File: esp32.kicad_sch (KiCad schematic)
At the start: 28 parts, among them U26 SRV05-4, U4 W25Q128, U5 ESP32-S3, Y1 40MHz

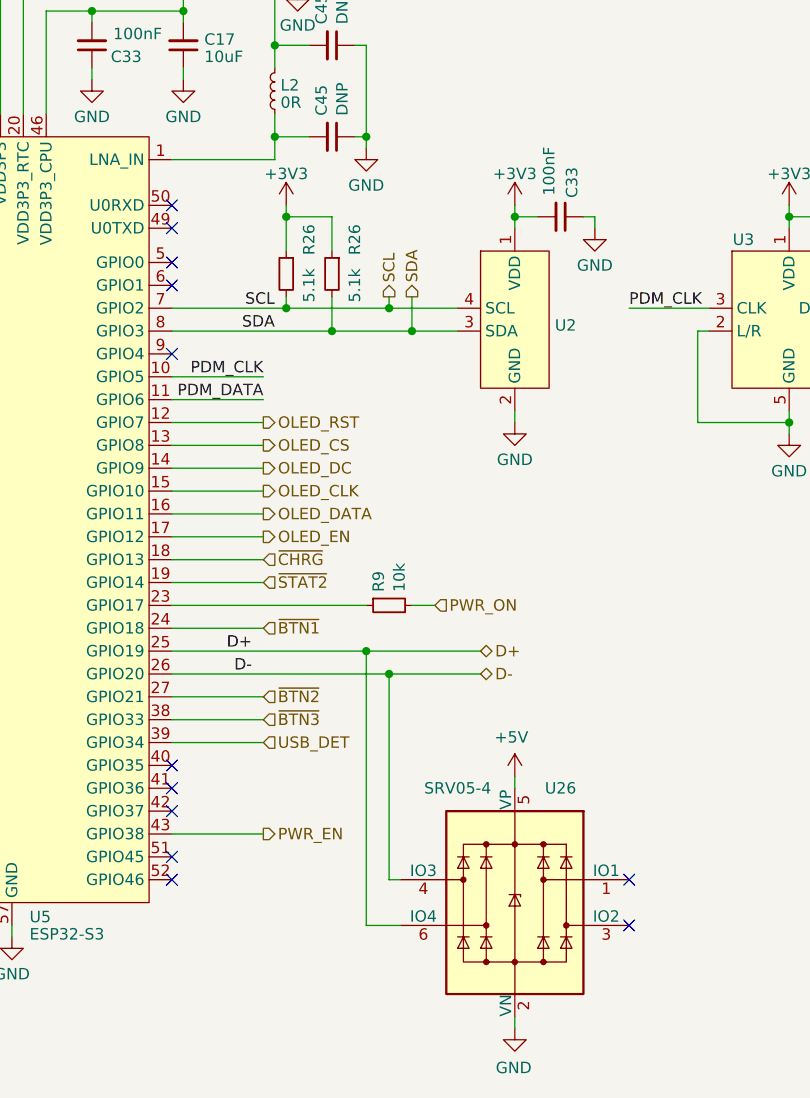
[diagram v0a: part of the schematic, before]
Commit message: Finish ESP32 fanout
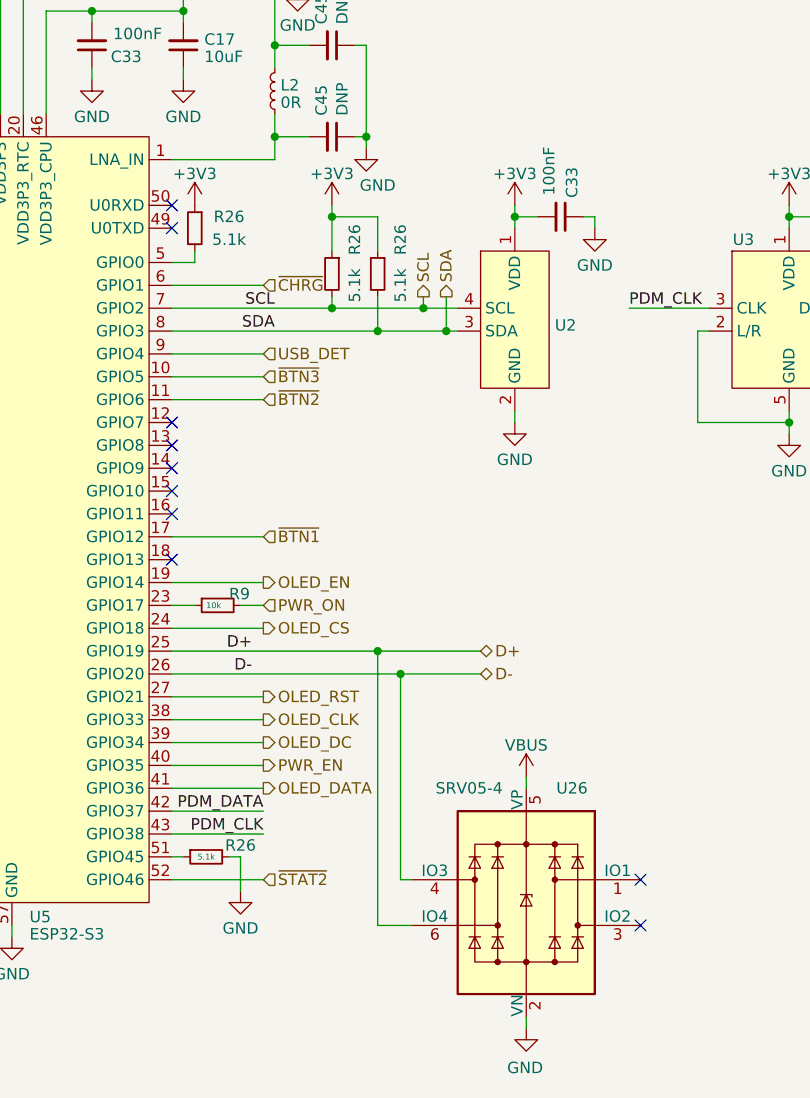
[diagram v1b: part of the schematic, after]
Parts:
- added R26 (x2): 5.1k, Resistor_SMD:R_0402_1005Metric, symbol Device:R_Small
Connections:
- net +3V3: now also R26.1
- net GND: now also R26.2
- net OLED_CLK: now also U5.38 (GPIO33); no longer U5.15 (GPIO10)
- net OLED_CS: now also U5.24 (GPIO18); no longer U5.13 (GPIO8)
- net OLED_DATA: now also U5.41 (GPIO36); no longer U5.16 (GPIO11)
- net OLED_DC: now also U5.39 (GPIO34); no longer U5.14 (GPIO9)
- net OLED_EN: now also U5.19 (GPIO14); no longer U5.17 (GPIO12)
- net OLED_RST: now also U5.27 (GPIO21); no longer U5.12 (GPIO7)
- net PDM_CLK: now also U5.43 (GPIO38); no longer U5.10 (GPIO5)
- net PDM_DATA: now also U5.42 (GPIO37); no longer U5.11 (GPIO6)
- net PWR_EN: now also U5.40 (GPIO35); no longer U5.43 (GPIO38)
- net USB_DET: now also U5.9 (GPIO4); no longer U5.39 (GPIO34)
- net ~{BTN1}: now also U5.17 (GPIO12); no longer U5.24 (GPIO18)
- net ~{BTN2}: now also U5.11 (GPIO6); no longer U5.27 (GPIO21)
- net ~{BTN3}: now also U5.10 (GPIO5); no longer U5.38 (GPIO33)
- net ~{CHRG}: now also U5.6 (GPIO1); no longer U5.18 (GPIO13)
- net ~{STAT2}: now also U5.52 (GPIO46); no longer U5.19 (GPIO14)
- net at U5.5 (GPIO0): now also R26.2
- net at U5.51 (GPIO45): now also R26.1
- net +5V renamed VBUS
- no-connect marks 21 -> 19
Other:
- moved on the sheet: R26, R9, U26
